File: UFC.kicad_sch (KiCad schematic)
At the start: 49 parts, among them M1 Fan_3pin, M2 Fan_3pin, M3 Fan_3pin, M4 Fan_3pin, M5 Fan_3pin, M6 Fan_3pin, M7 Fan_3pin, M8 Fan_3pin, U1 Pico

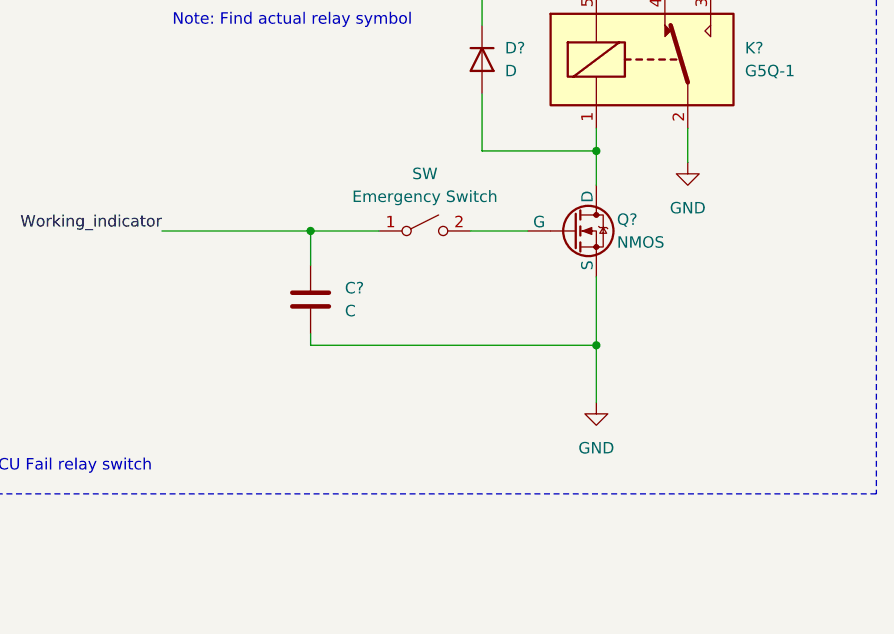
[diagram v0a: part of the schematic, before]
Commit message: Tweak relay circuit
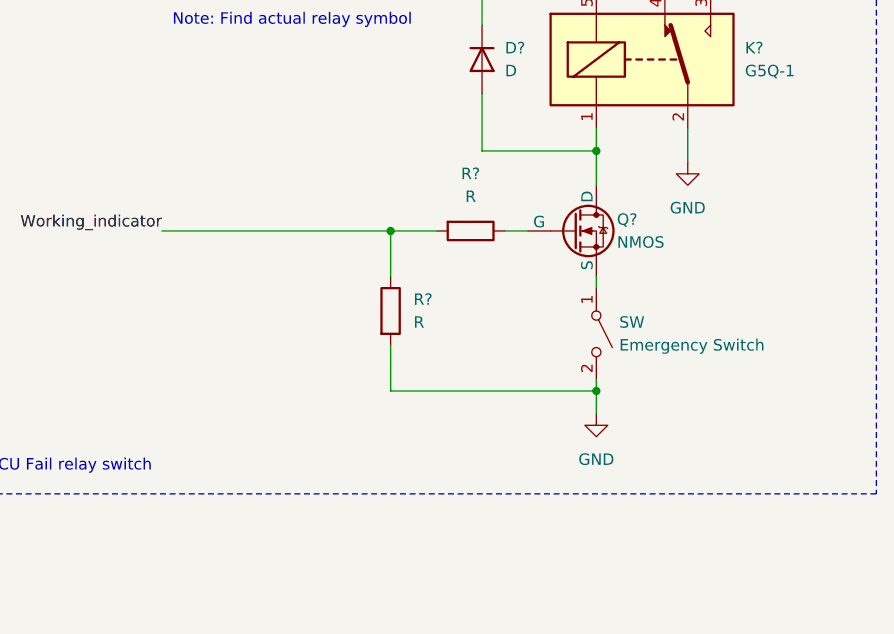
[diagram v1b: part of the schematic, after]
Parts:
- removed C?: C, symbol Device:C
- added R? (x2): R, symbol Device:R
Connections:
- net GND: now also SW.2 (B), R?.2; no longer Q?.3 (S)
- net Working_indicator: now also R?.1, R?.2; no longer SW.1 (A)
- net at Q?.2 (G): now also R?.1; no longer SW.2 (B)
- new net: Q?.3 (S), SW.1 (A)
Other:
- moved on the sheet: SW
